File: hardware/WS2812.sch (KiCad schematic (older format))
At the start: 38 parts

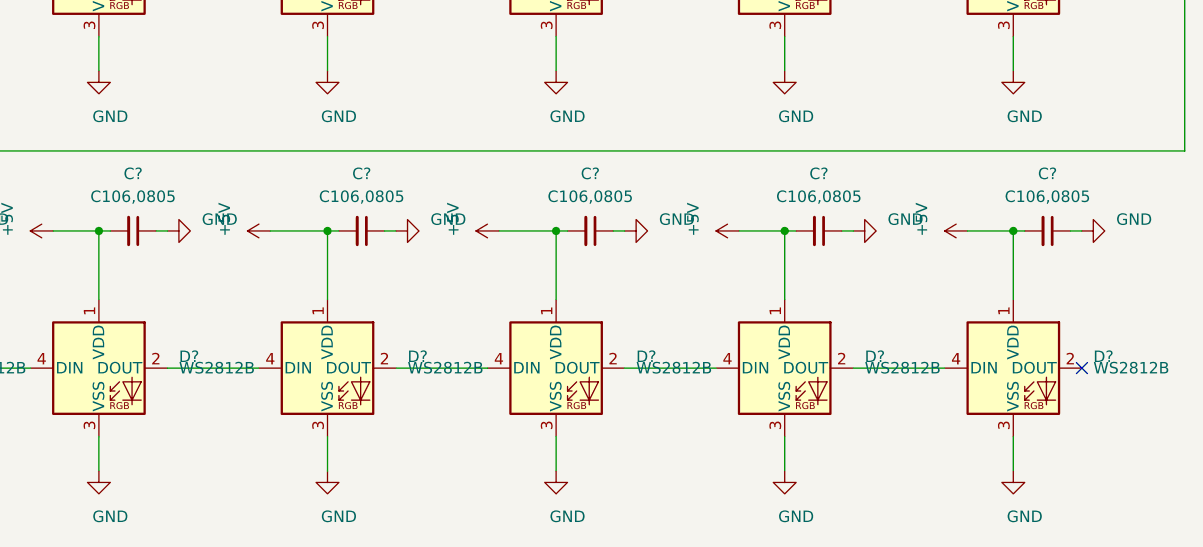
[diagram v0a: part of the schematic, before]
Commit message: update for cherry key,
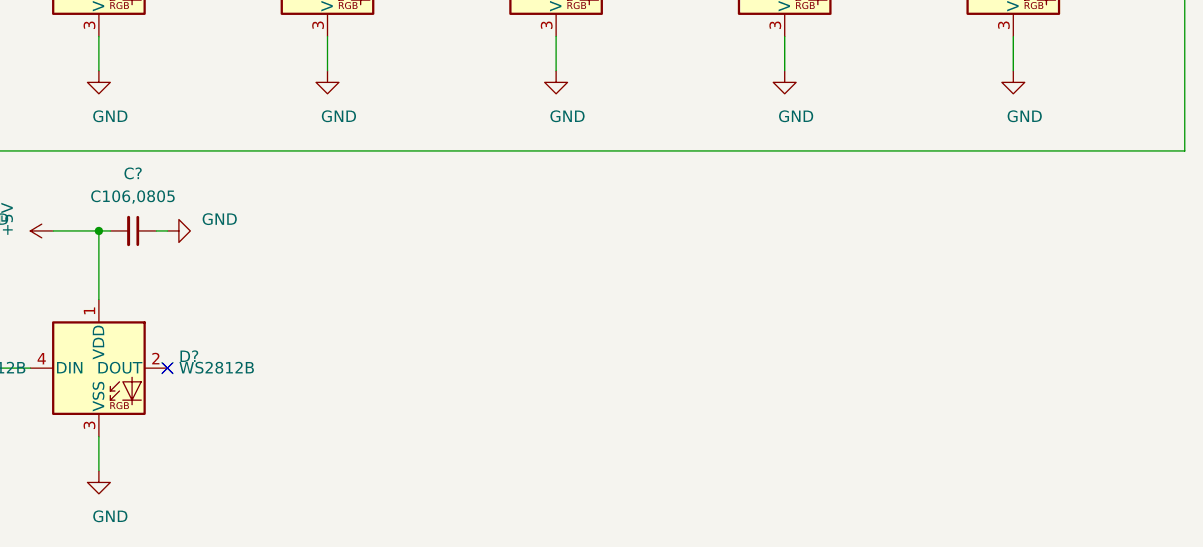
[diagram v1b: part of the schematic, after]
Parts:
- removed C? (x4): C106,0805, Capacitor_SMD:C_0805_2012Metric_Pad1.15x1.40mm_HandSolder, symbol taobao-c:C106,0805
- removed D? (x4): WS2812B, LED_SMD:LED_WS2812B_PLCC4_5.0x5.0mm_P3.2mm, symbol LED:WS2812B
